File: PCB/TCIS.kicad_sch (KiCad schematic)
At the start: 9 parts, among them U1 NE555P

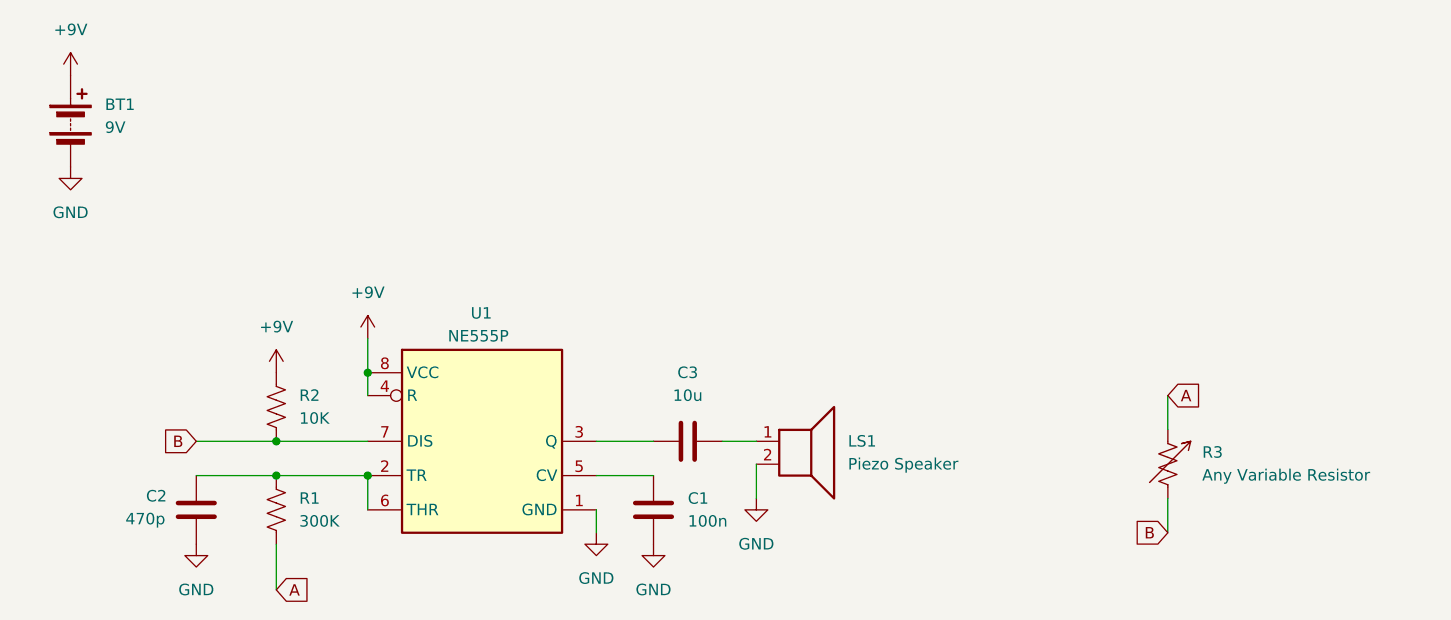
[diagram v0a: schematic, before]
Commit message: Updated PCB
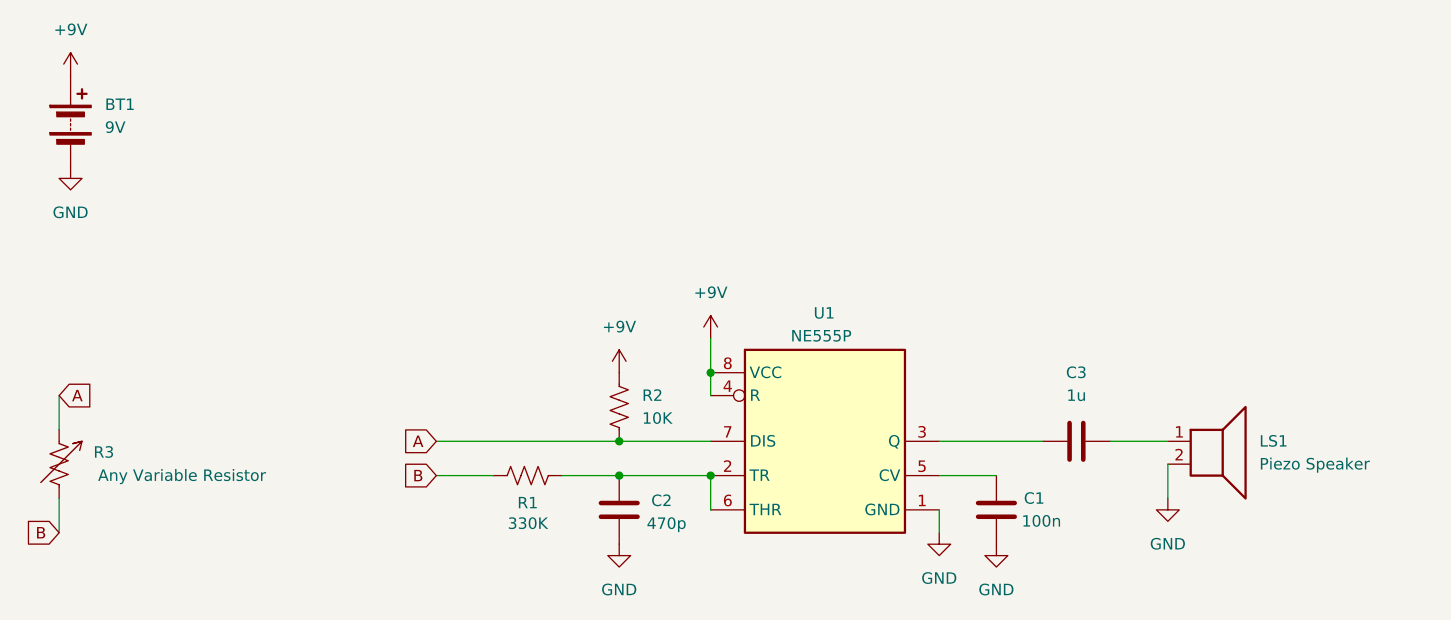
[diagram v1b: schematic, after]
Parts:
- C3: value 10u -> 1u
- R1: value 300K -> 330K
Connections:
- net A: now also R2.2, U1.7 (DIS); no longer R1.2
- net B: now also R1.2; no longer R2.2, U1.7 (DIS)
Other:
- moved on the sheet: C1, C2, C3, LS1, R1, R2, R3, U1
